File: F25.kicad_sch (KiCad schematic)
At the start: 37 parts, among them J3 B2B-PH-K-S, J4 USB_C_Receptacle_USB2.0_16P, Q1 IRLML6244, SW1 RESET, SW2 BOOT, U2 MPU-6050, U3 MS5611-01BA, U4 ESP32-S3-WROOM-1-N8, U5 AP2112K-3.3

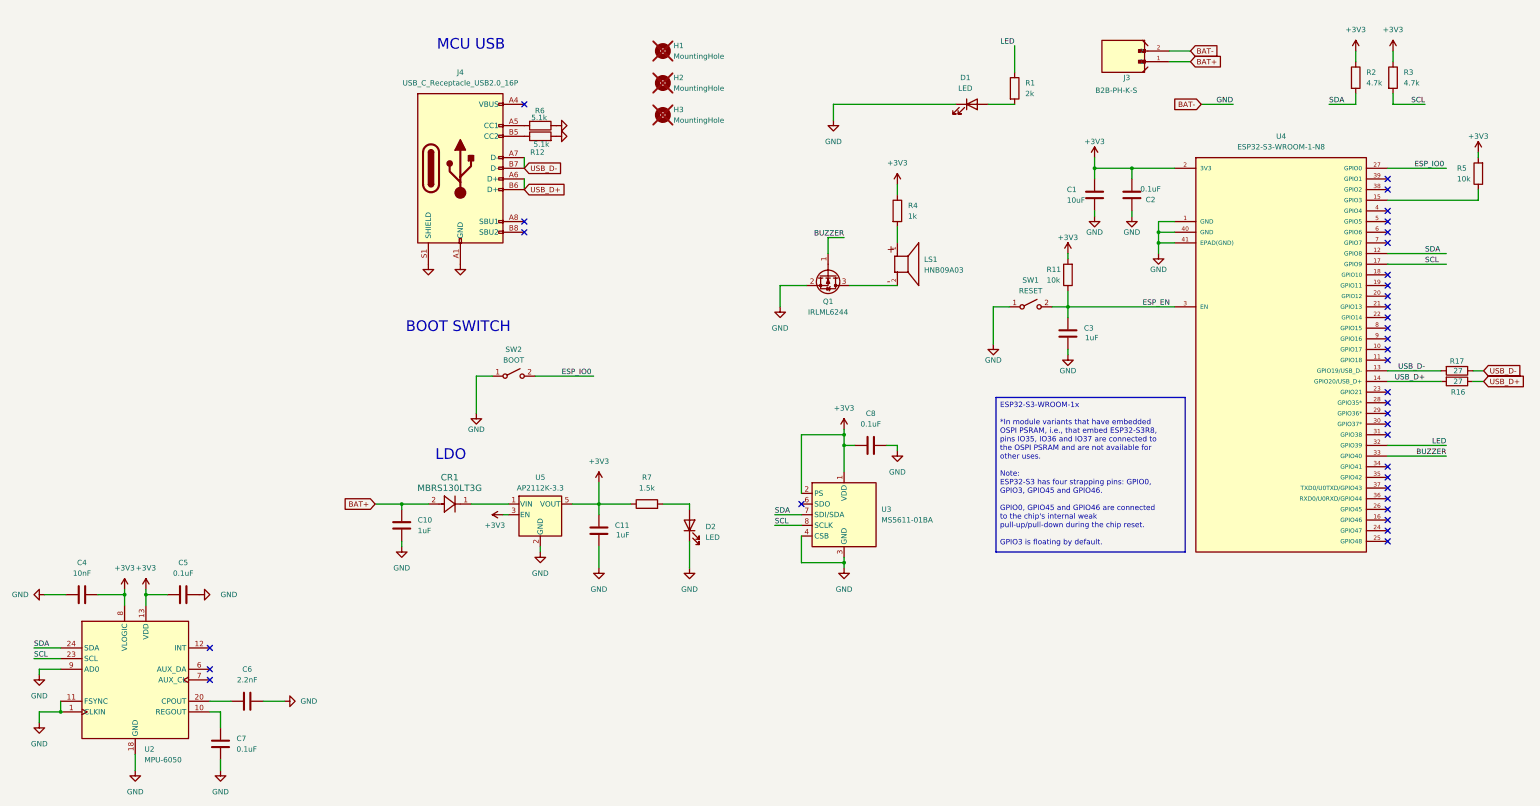
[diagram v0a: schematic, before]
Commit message: General Updates
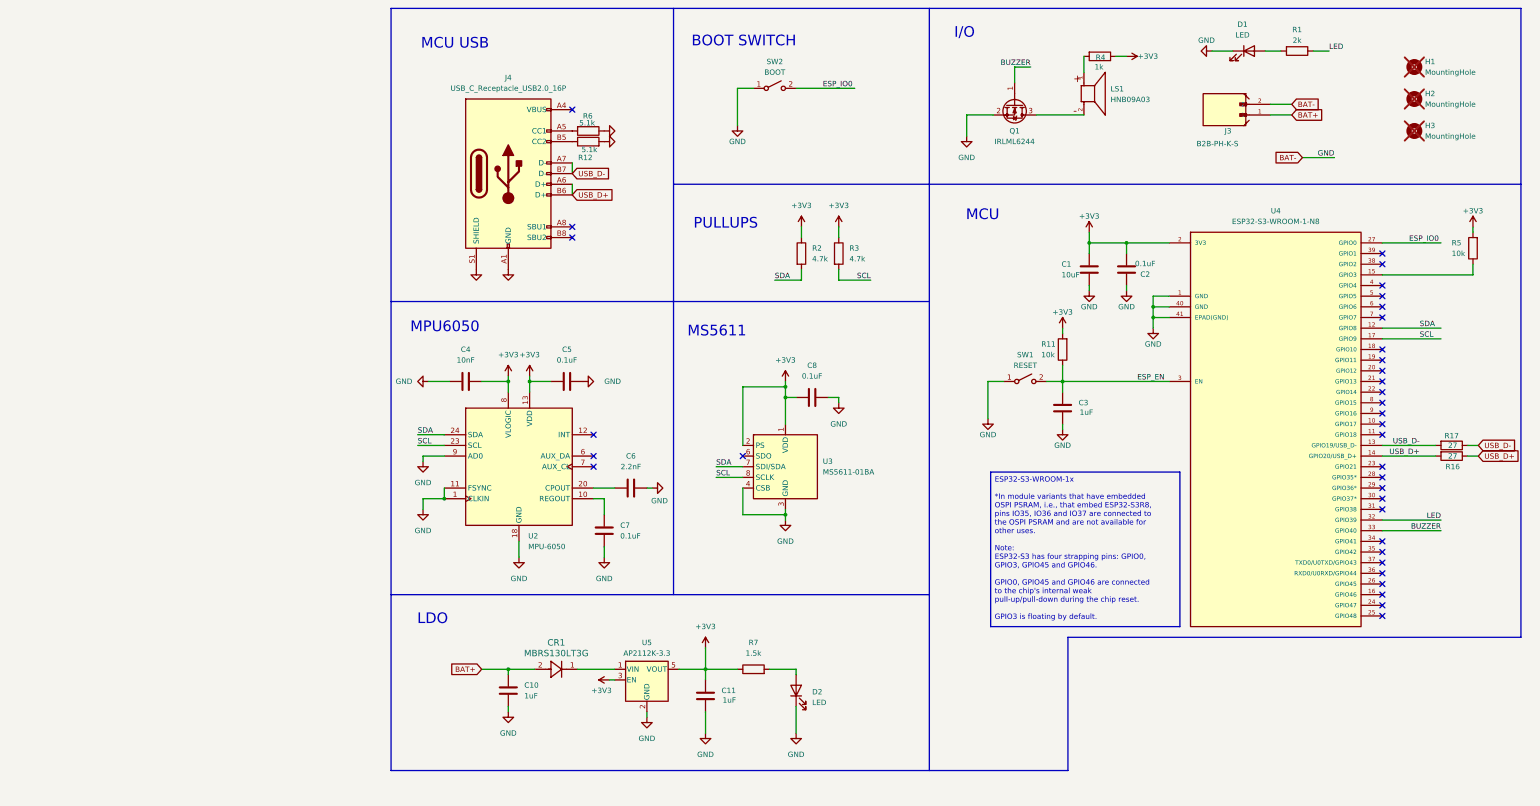
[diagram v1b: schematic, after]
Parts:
- U4: footprint ESP:ESP32-S3-WROOM-1_EXP -> RF_Module:ESP32-S3-WROOM-1
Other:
- note added: "I/O"
- note added: "MCU"
- note added: "MPU6050"
- note added: "MS5611"
- note added: "PULLUPS"
- title: Eggtimer Ion Flight Computer  -> MARS F25 Board
- moved on the sheet: C1, C10, C11, C2, C3, C4, C5, C6, C7, C8, CR1, D1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
